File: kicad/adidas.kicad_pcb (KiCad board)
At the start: 2 copper layers, 2 parts

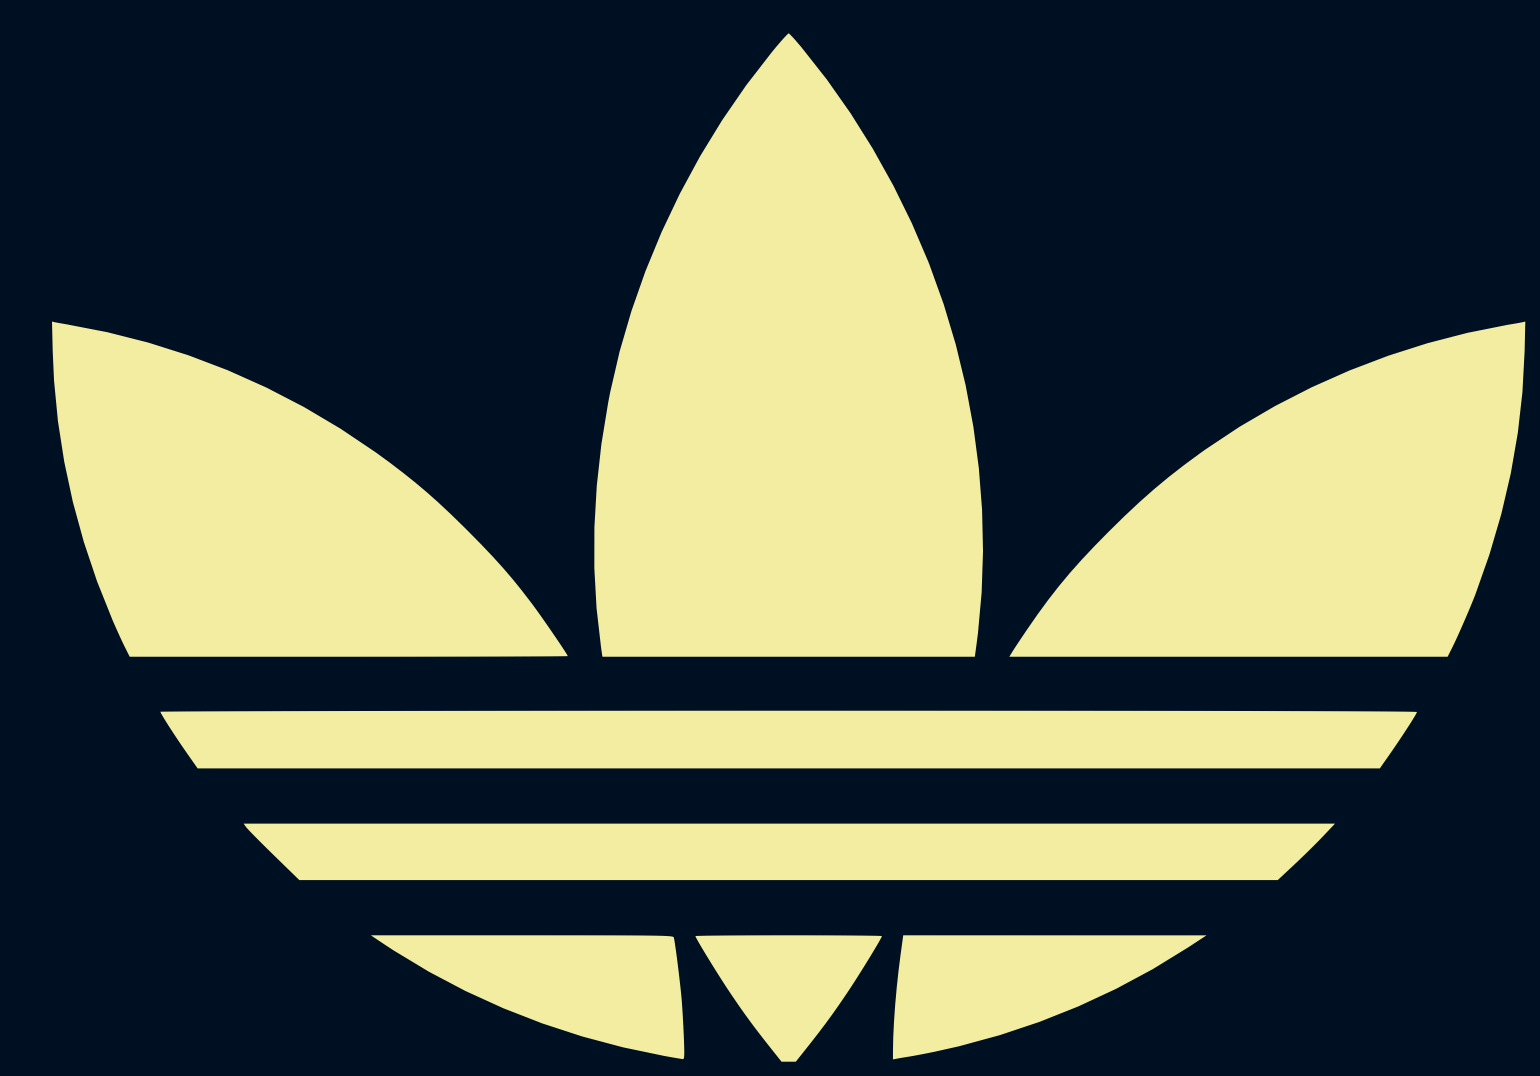
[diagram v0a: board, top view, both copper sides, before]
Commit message: v0.1
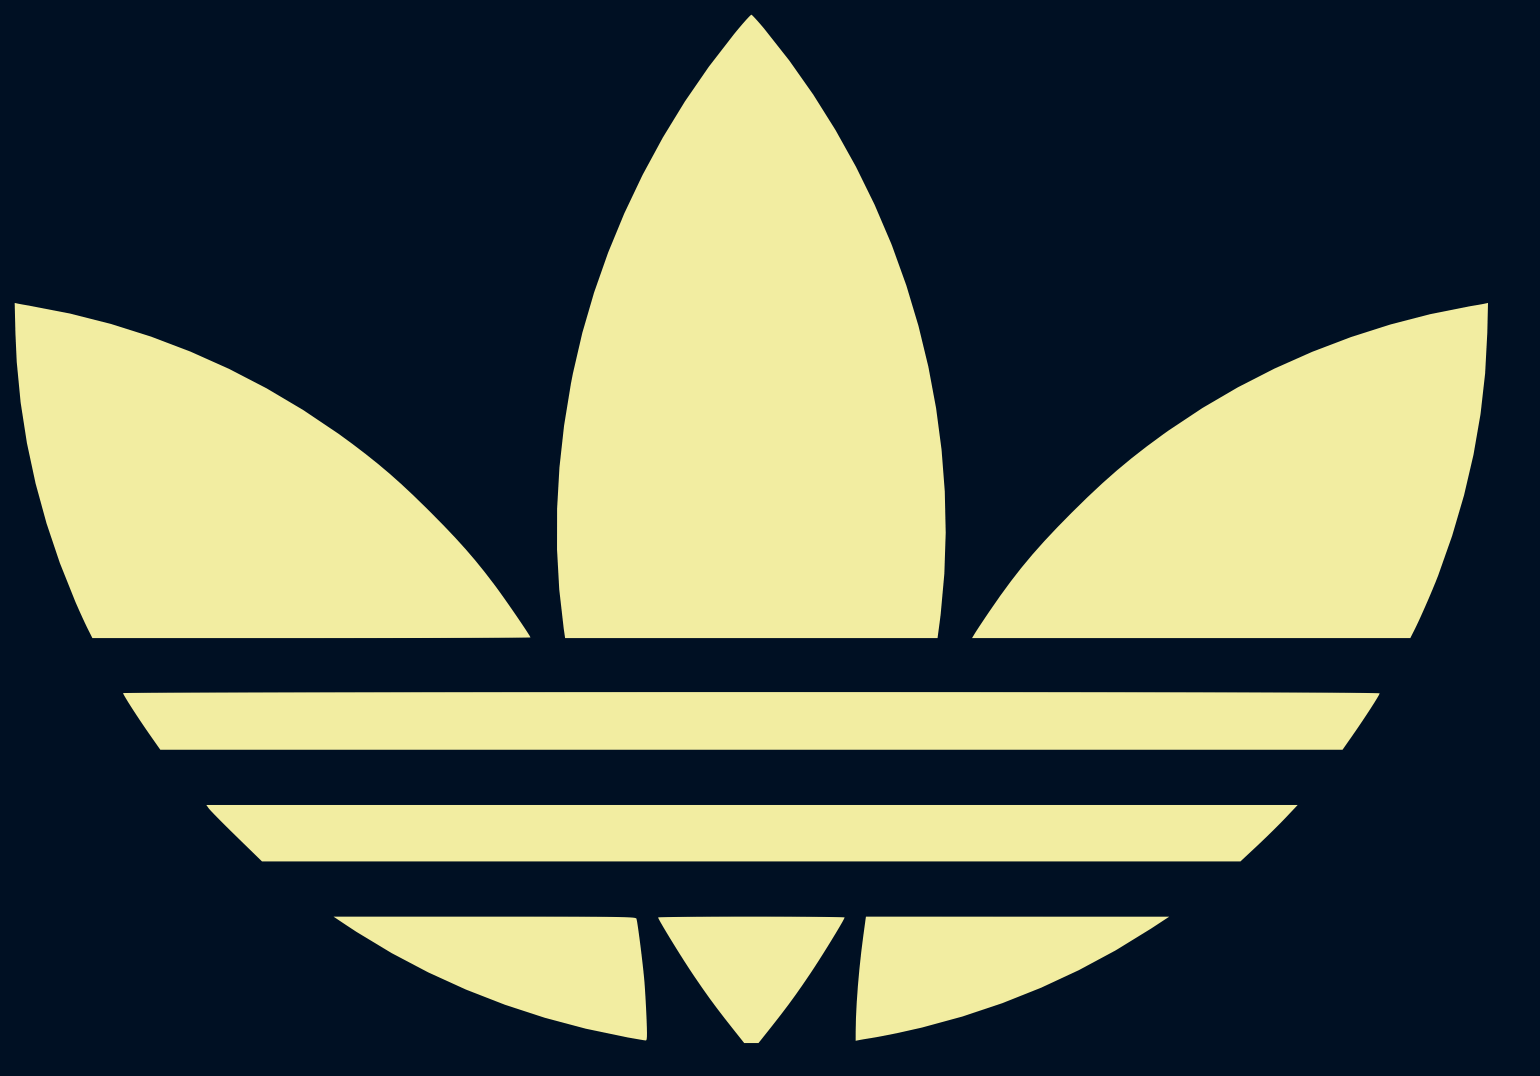
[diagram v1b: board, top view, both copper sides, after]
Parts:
- removed the G*** at (152.4, 96.5)
- added G***: LOGO, DEAD10C5:Adidas, F.Cu at (147.3, 94.0)
- moved G*** 69.7 mm to (221.0, 91.4)
